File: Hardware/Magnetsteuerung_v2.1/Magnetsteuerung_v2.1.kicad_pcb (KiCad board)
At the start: 2 copper layers, 92.1 x 100.1 mm, 190 parts, among them J1 Conn_02x08_Odd_Even, J3 Conn_01x16, J9 Conn_01x16, Q1 Q_NMOS_GSD, Q10 Q_NMOS_GSD, Q11 Q_NMOS_GSD, Q12 Q_NMOS_GSD, Q13 Q_NMOS_GSD, Q14 Q_NMOS_GSD, Q15 Q_NMOS_GSD, Q16 Q_NMOS_GSD, Q17 Q_NMOS_GDS, Q2 Q_NMOS_GSD, Q3 Q_NMOS_GSD, Q4 Q_NMOS_GSD, Q5 Q_NMOS_GSD, Q6 Q_NMOS_GSD, Q7 Q_NMOS_GSD, Q8 Q_NMOS_GSD, U1 TL2575, U10 MCP1416R, U11 MCP1416R, U12 MCP1416R, U13 MCP1416R, U14 MCP1416R, U15 MCP1416R, U16 MCP1416R, U17 MCP1416R, U2 MCP1416R, U3 MCP1416R, U4 MCP1416R, U5 MCP1416R, U6 MCP1416R, U7 MCP1416R, U8 MCP1416R, U9 MCP1416R

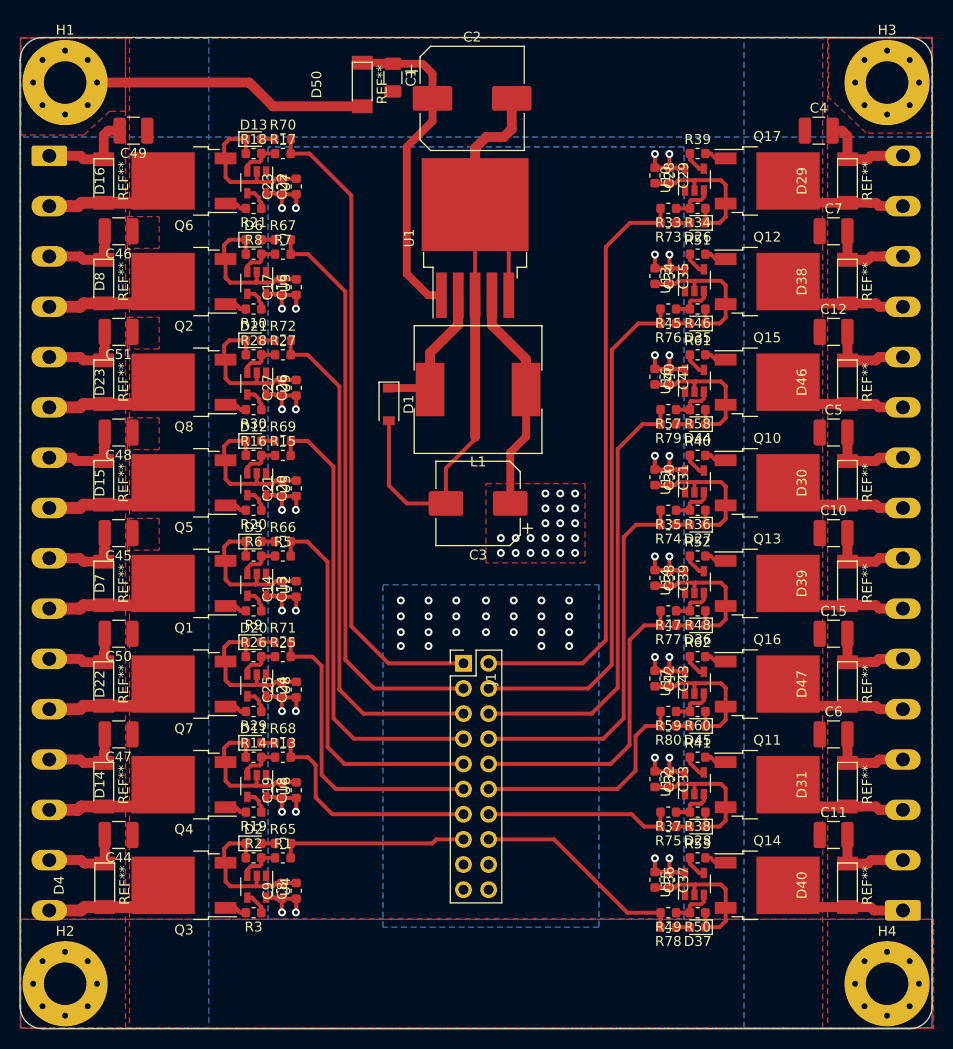
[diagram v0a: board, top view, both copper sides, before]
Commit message: fertigungsdaten aufbereitet
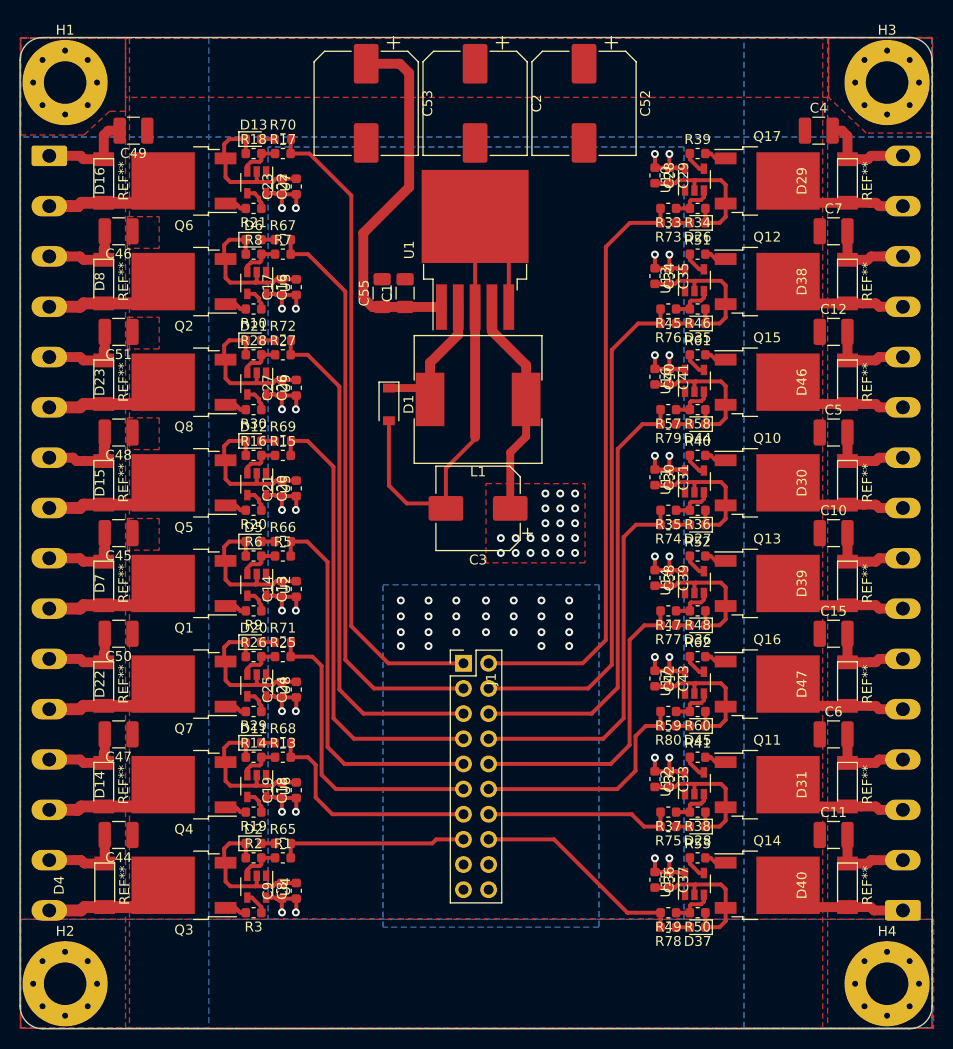
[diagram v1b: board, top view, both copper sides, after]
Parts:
- removed D50: PMEG6010CEH, MK_Footprints:D_SOD_128_2
- added C52: 100u, Capacitor_SMD:CP_Elec_10x10, F.Cu at (145.9, 37.6)
- added C53: 100u, Capacitor_SMD:CP_Elec_10x10, F.Cu at (123.9, 37.6)
- added C55: 100n, Capacitor_SMD:C_1206_3216Metric, F.Cu at (125.5, 56.8)
- moved C1 21.8 mm to (127.8, 56.8), turned to 90 degrees
- moved U1 1.20 mm to (134.9, 52.4)
- moved L1 1.00 mm to (135.2, 67.5)
- moved C2 0.58 mm to (134.9, 37.6), turned to 270 degrees
- moved C3 0.50 mm to (135.2, 78.5)
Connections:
- C1 pad 1: Net-(C1-Pad1) -> +48V
- C2 pad 1: Net-(C1-Pad1) -> +48V
- U1 pad 1: Net-(C1-Pad1) -> +48V
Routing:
- net Net-(C1-Pad1): track 33.2 -> 0.00 mm
- net GND: track 319.2 -> 305.9 mm
- net +48V: track 177.4 -> 184.0 mm
- net Net-(D1-Pad1): track 19.1 -> 21.3 mm
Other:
- board text added: "Pamatech System AG"
- board text added: "SN4855S24A8"
- board text added: "Vin: 48-55V"
- board text removed: "+48V"

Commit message: change hardware
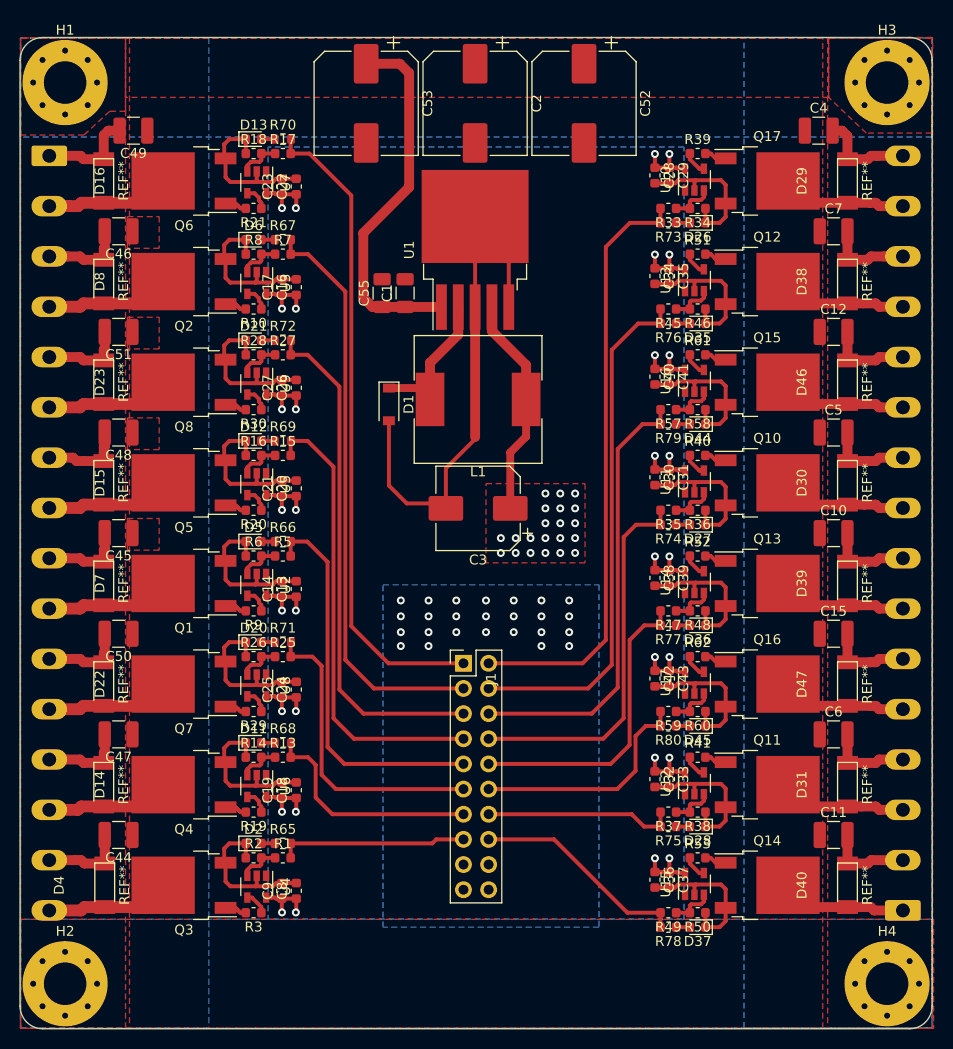
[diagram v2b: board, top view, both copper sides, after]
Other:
- net class Default removed
